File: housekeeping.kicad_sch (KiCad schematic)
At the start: 3 parts, among them U4 TPS7B8133QDGNRQ1

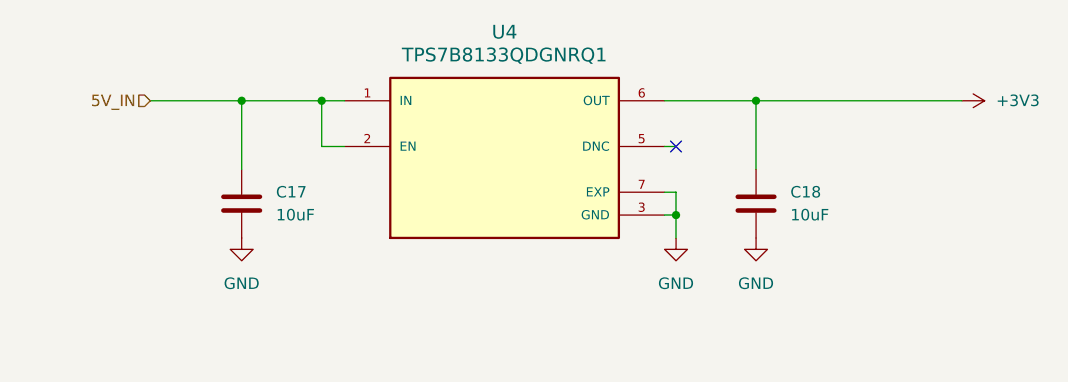
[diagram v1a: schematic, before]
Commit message: Updating stuff
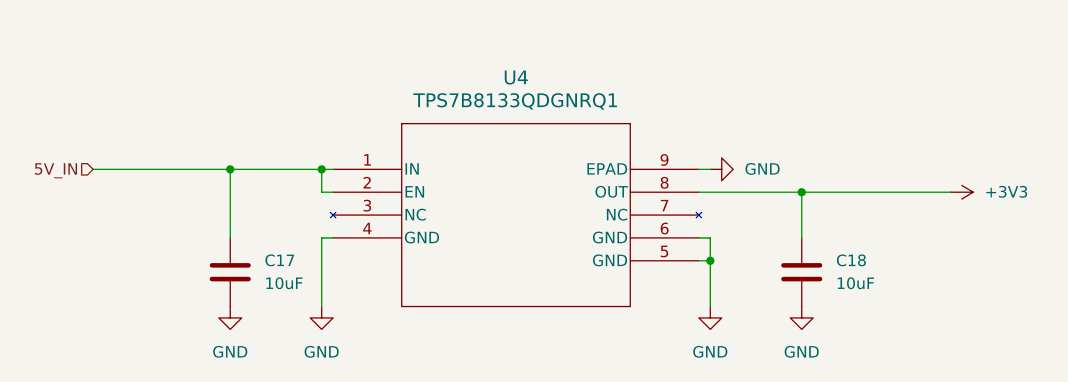
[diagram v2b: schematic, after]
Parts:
- removed U4: TPS7B8133QDGNRQ1, _BMS:VSSOP8_DGN_TEX, symbol _TPS7B:TPS7B8133DRVR
- added U4: TPS7B8133QDGNRQ1, VSSOP8_DGN_TEX, symbol _TPS7B:TPS7B8133QDGNRQ1
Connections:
- net +3V3: now also U4.8 (OUT)
- net 5V_IN: now also U4.1 (IN), U4.2 (EN)
- net GND: now also U4.4 (GND), U4.5 (GND), U4.6 (GND), U4.9 (EPAD)
- no-connect marks 1 -> 0
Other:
- moved on the sheet: C17, C18

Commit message: Placement
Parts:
- U4: footprint VSSOP8_DGN_TEX -> _BMS:VSSOP8_DGN_TEX
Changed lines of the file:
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@@
 		(dnp no)
 		(fields_autoplaced yes)
-		(property "Reference" "#PWR072"
+		(property "Reference" "#PWR048"
 			(at 175.26 99.06 0)
 			(effects
@@
 			(project "BMS"
 				(path "/124184ba-5d68-4d9f-8da6-acc6720ab30b/93f9b420-7cce-46a9-9201-666f07a18f85/1875dae8-5675-4324-bc32-eabf0e306a05"
-					(reference "#PWR072")
+					(reference "#PWR048")
 					(unit 1)
 				)
@@
 		(dnp no)
 		(fields_autoplaced yes)
-		(property "Reference" "#PWR048"
+		(property "Reference" "#PWR046"
 			(at 115.57 120.65 0)
 			(effects
@@
 			(project ""
 				(path "/124184ba-5d68-4d9f-8da6-acc6720ab30b/93f9b420-7cce-46a9-9201-666f07a18f85/1875dae8-5675-4324-bc32-eabf0e306a05"
-					(reference "#PWR048")
+					(reference "#PWR046")
 					(unit 1)
 				)
@@
 			)
 		)
-		(property "Footprint" "VSSOP8_DGN_TEX"
+		(property "Footprint" "_BMS:VSSOP8_DGN_TEX"
 			(at 127 99.06 0)
 			(effects
@@
 		(dnp no)
 		(fields_autoplaced yes)
-		(property "Reference" "#PWR071"
+		(property "Reference" "#PWR047"
 			(at 125.73 120.65 0)
 			(effects
@@
 			(project "BMS"
 				(path "/124184ba-5d68-4d9f-8da6-acc6720ab30b/93f9b420-7cce-46a9-9201-666f07a18f85/1875dae8-5675-4324-bc32-eabf0e306a05"
-					(reference "#PWR071")
+					(reference "#PWR047")
 					(unit 1)
 				)
